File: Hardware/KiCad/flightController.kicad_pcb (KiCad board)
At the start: 4 copper layers, 57 x 57 mm, 183 parts, among them J1 USB_B_Mini, J10 JST SH1-2P, J11 MOLEX 5268-7P, J12 JST SH1-8P, J2 USB_B_Mini, J3 2.54mm header, J4 2.54mm header, J5 TF-01A, J6 1mm header, J7 JST SH1-4P, J8 JST SH1-4P, J9 JST SH1-4P, Q1 PMBT3904, Q2 PMBT3904, SW1 SW_SPDT, SW2 SW_Push, U1 MPU-6000, U10 CH330N, U11 SMF05CT1G, U12 SMF05CT1G, U13 SMF05CT1G, U2 HMC5883L, U3 FM24C64B, U4 BMP388, U5 STM32H743VIT6, U6 AMS1117-5V, U7 AMS1117-3.3, U8 SMF05CT1G, U9 SMF05CT1G

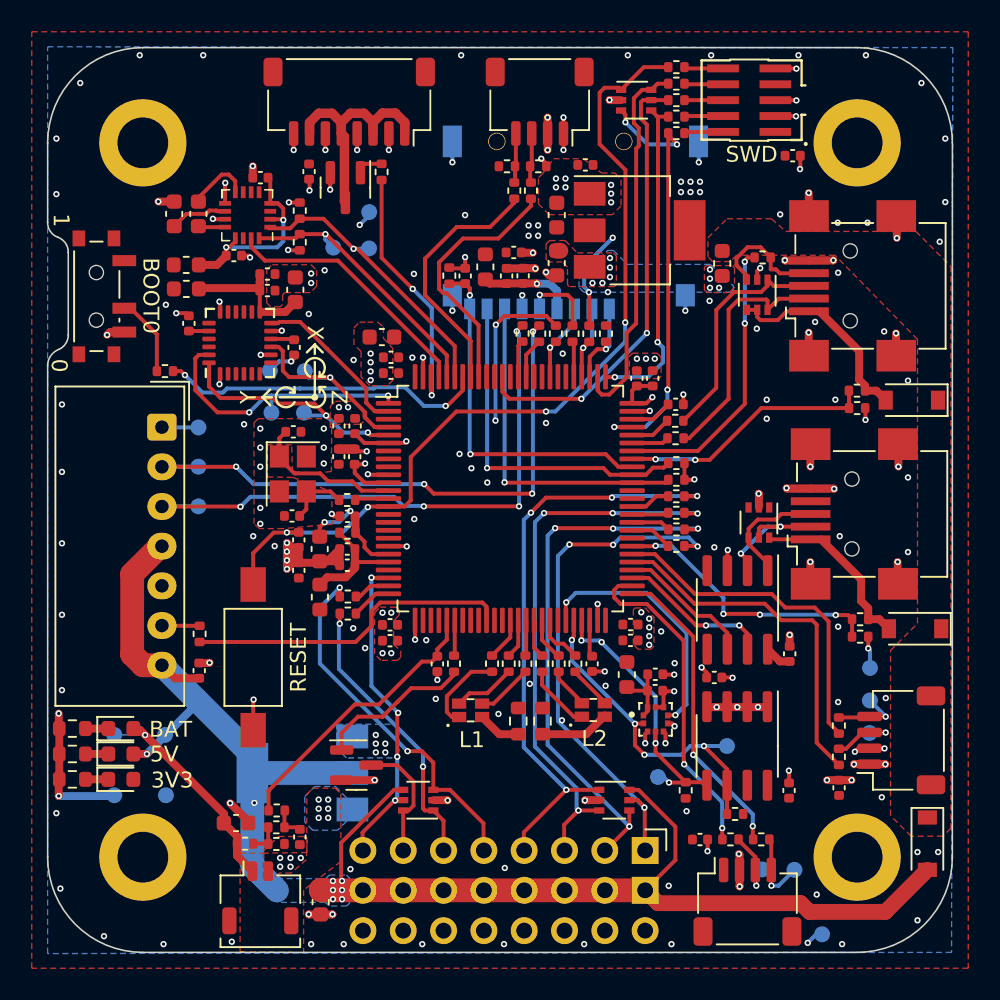
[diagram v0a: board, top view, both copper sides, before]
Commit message: Added labels
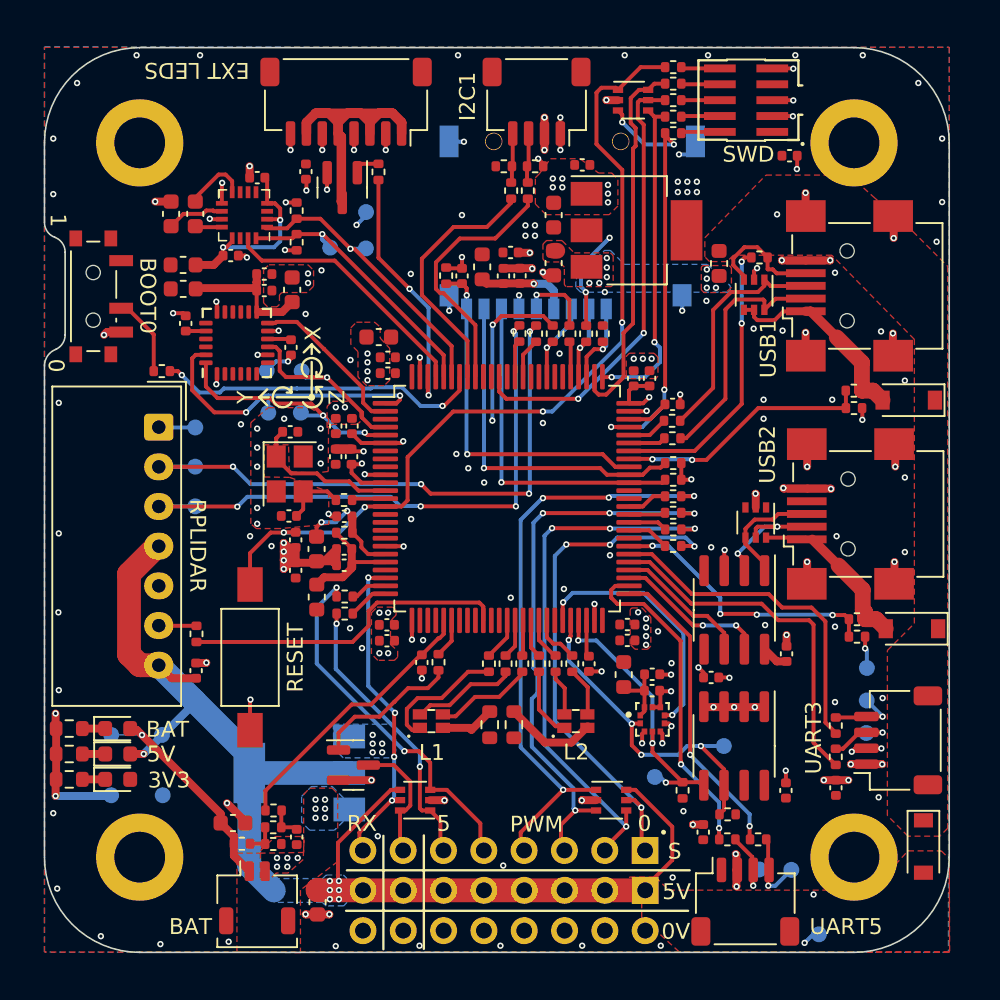
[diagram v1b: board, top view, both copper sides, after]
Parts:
- moved D1 2.56 mm to (94.4, 119.5)
- moved R2 1.81 mm to (98.0, 119.7), turned to 90 degrees
- moved R6 1.81 mm to (99.6, 119.7), turned to 90 degrees
- moved D2 1.30 mm to (103.5, 119.5)
- moved C14 0.98 mm to (93.8, 115.8)
- moved R16 0.98 mm to (94.8, 115.7)
- moved C50 0.51 mm to (111.5, 126.4), turned to 90 degrees
- moved R42 0.47 mm to (113.0, 125.3)
- moved D6 0.31 mm to (125.4, 127.3)
- moved J2 0.24 mm to (120.6, 106.4)
- moved C10 0.20 mm to (116.7, 123.8)
- moved C12 0.20 mm to (108.3, 116.5)
- moved C13 0.20 mm to (85.9, 126.8)
- moved C15 0.20 mm to (104.3, 115.8)
- moved C16 0.20 mm to (109.6, 99.5)
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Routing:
- net +5V: track 97.2 -> 77.7 mm
- net Net-(J12-Pad1): track 14.7 -> 20.3 mm
- net Net-(D1-Pad2): track 3.96 -> 6.76 mm
- net Net-(D1-Pad3): track 3.56 -> 6.29 mm
- net Net-(D1-Pad1): track 5.39 -> 8.05 mm
- net IMU_SCL: track 17.7 -> 19.4 mm
- net Net-(D2-Pad4): track 4.66 -> 5.88 mm
- net GND: track 113.8 -> 112.6 mm
- net Net-(D1-Pad4): track 2.72 -> 3.48 mm
- net Net-(Q1-Pad1): track 9.87 -> 9.27 mm
- net +3V3: vias 115 -> 104
- added copper zone on F.Cu, net +5V
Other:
- outline, holes or cut-outs redrawn
- board text added: "RPLIDAR"

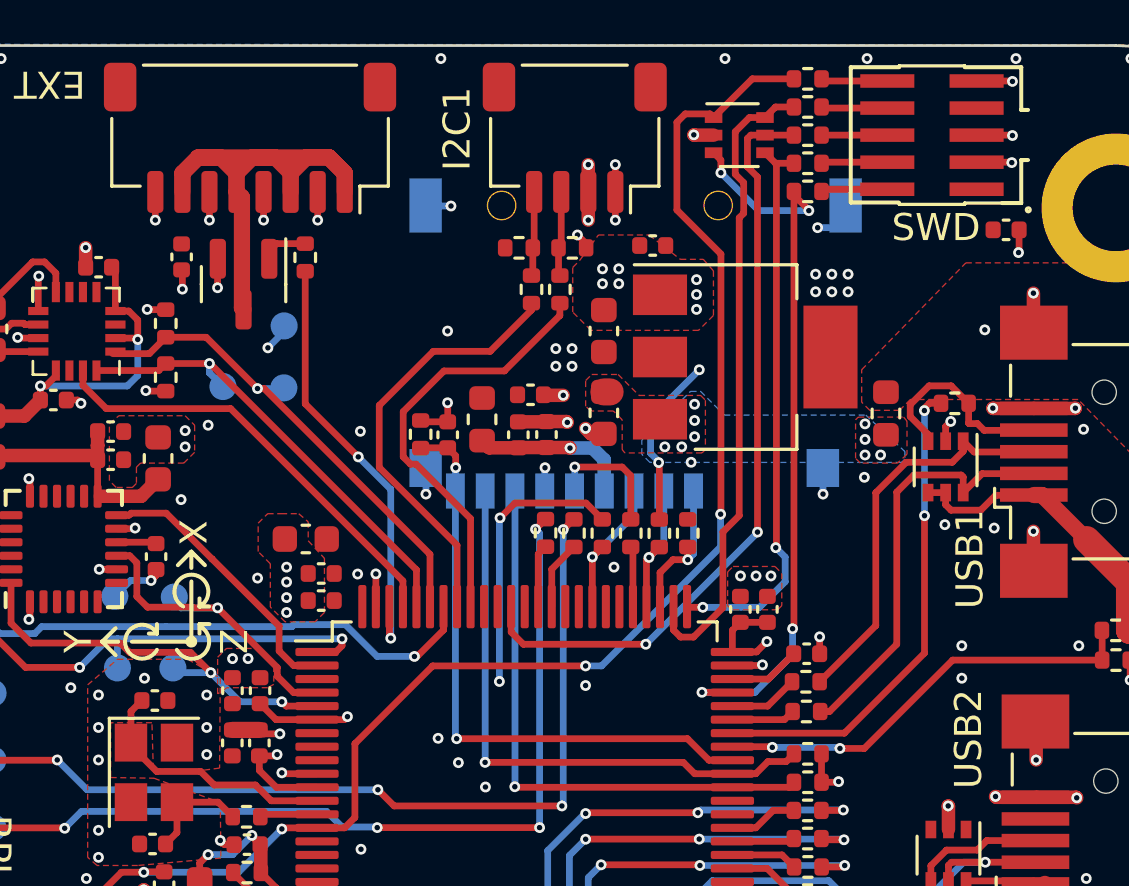
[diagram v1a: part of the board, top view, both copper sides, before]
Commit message: Layout optimizations
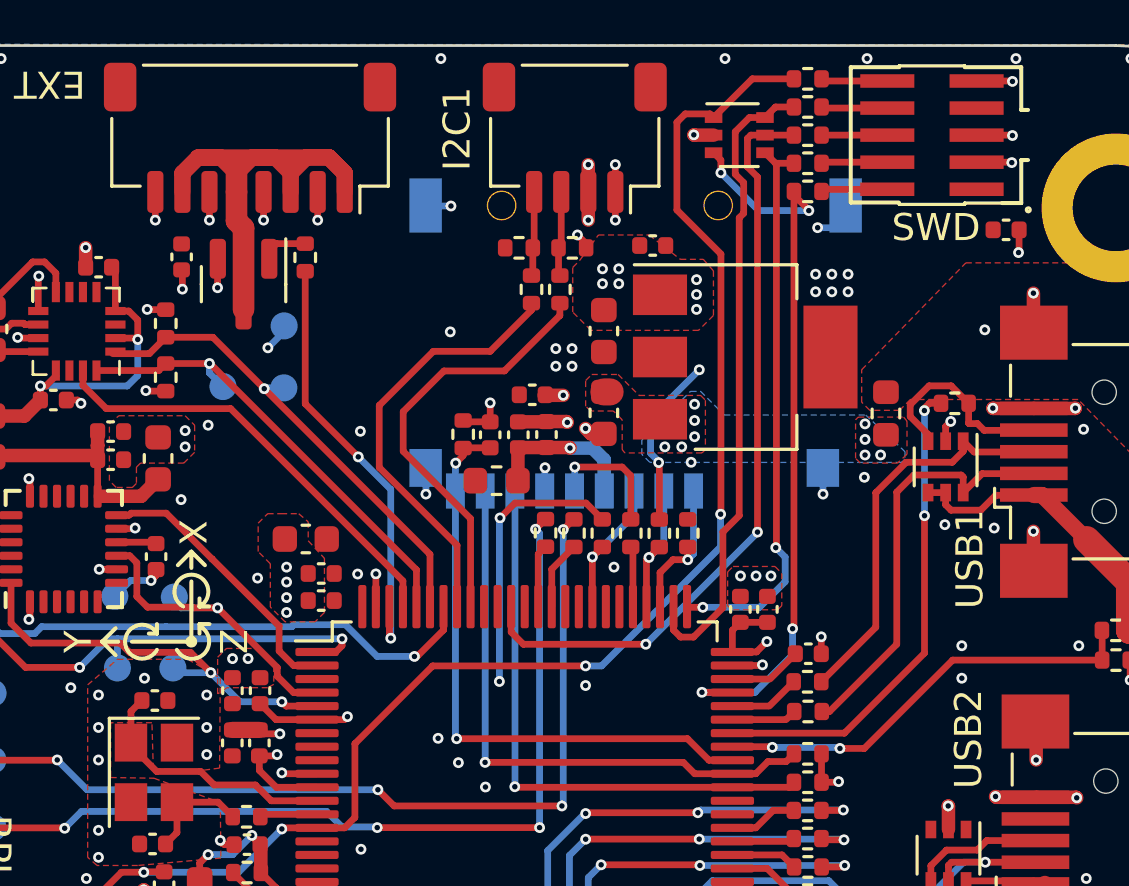
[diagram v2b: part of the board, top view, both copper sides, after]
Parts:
- moved FB6 2.33 mm to (98.1, 93.1), turned to 0 degrees
- moved C46 1.57 mm to (97.9, 91.4)
- moved R59 1.57 mm to (96.9, 91.4)
- moved C43 0.07 mm to (99.4, 89.9)
- moved C16 0.06 mm to (109.6, 99.5)
- moved R28 0.06 mm to (109.6, 101.6)
- moved R29 0.06 mm to (109.6, 100.5)
